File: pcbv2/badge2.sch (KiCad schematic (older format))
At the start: 25 parts, among them J1 Conn_02x04_Counter_Clockwise, J2 SAO_CONN, J3 USB_C_Receptacle_USB2.0, J6 Conn_ARM_JTAG_SWD_10, Q2 Si1308EDL, U3 E73-2G4M08S1C, U5 GD25Q16C, U7 LIS2DH12TR

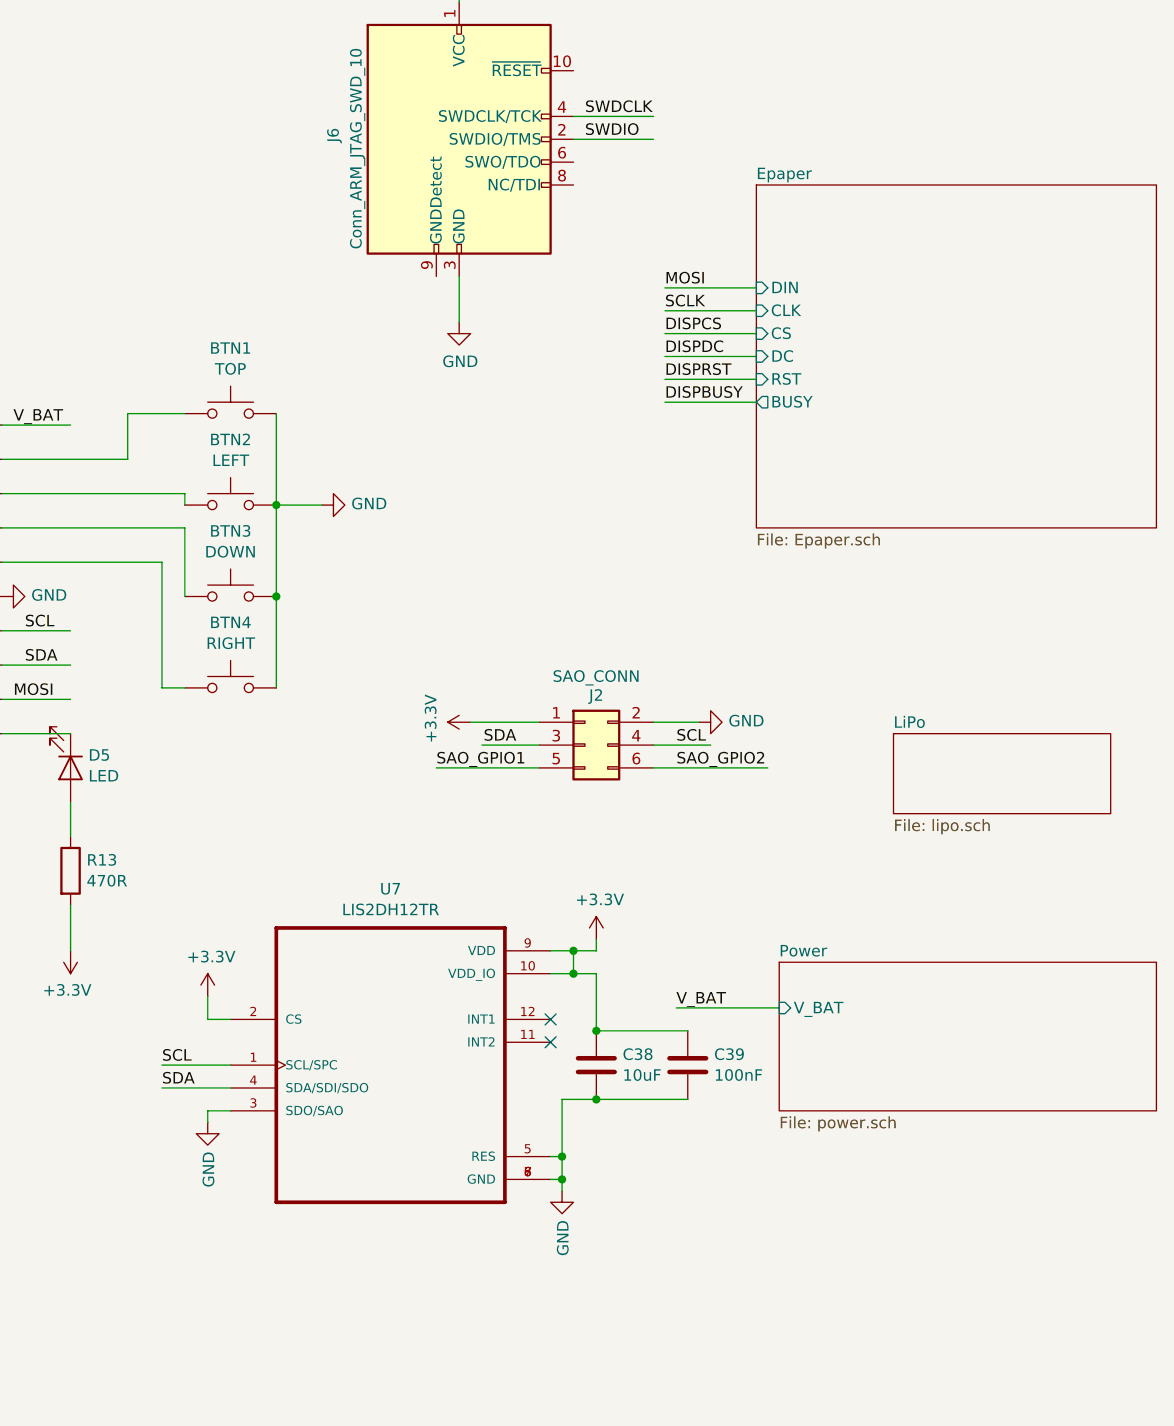
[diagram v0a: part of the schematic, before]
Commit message: refactor(pcbv2): move accelerometer to own sheet
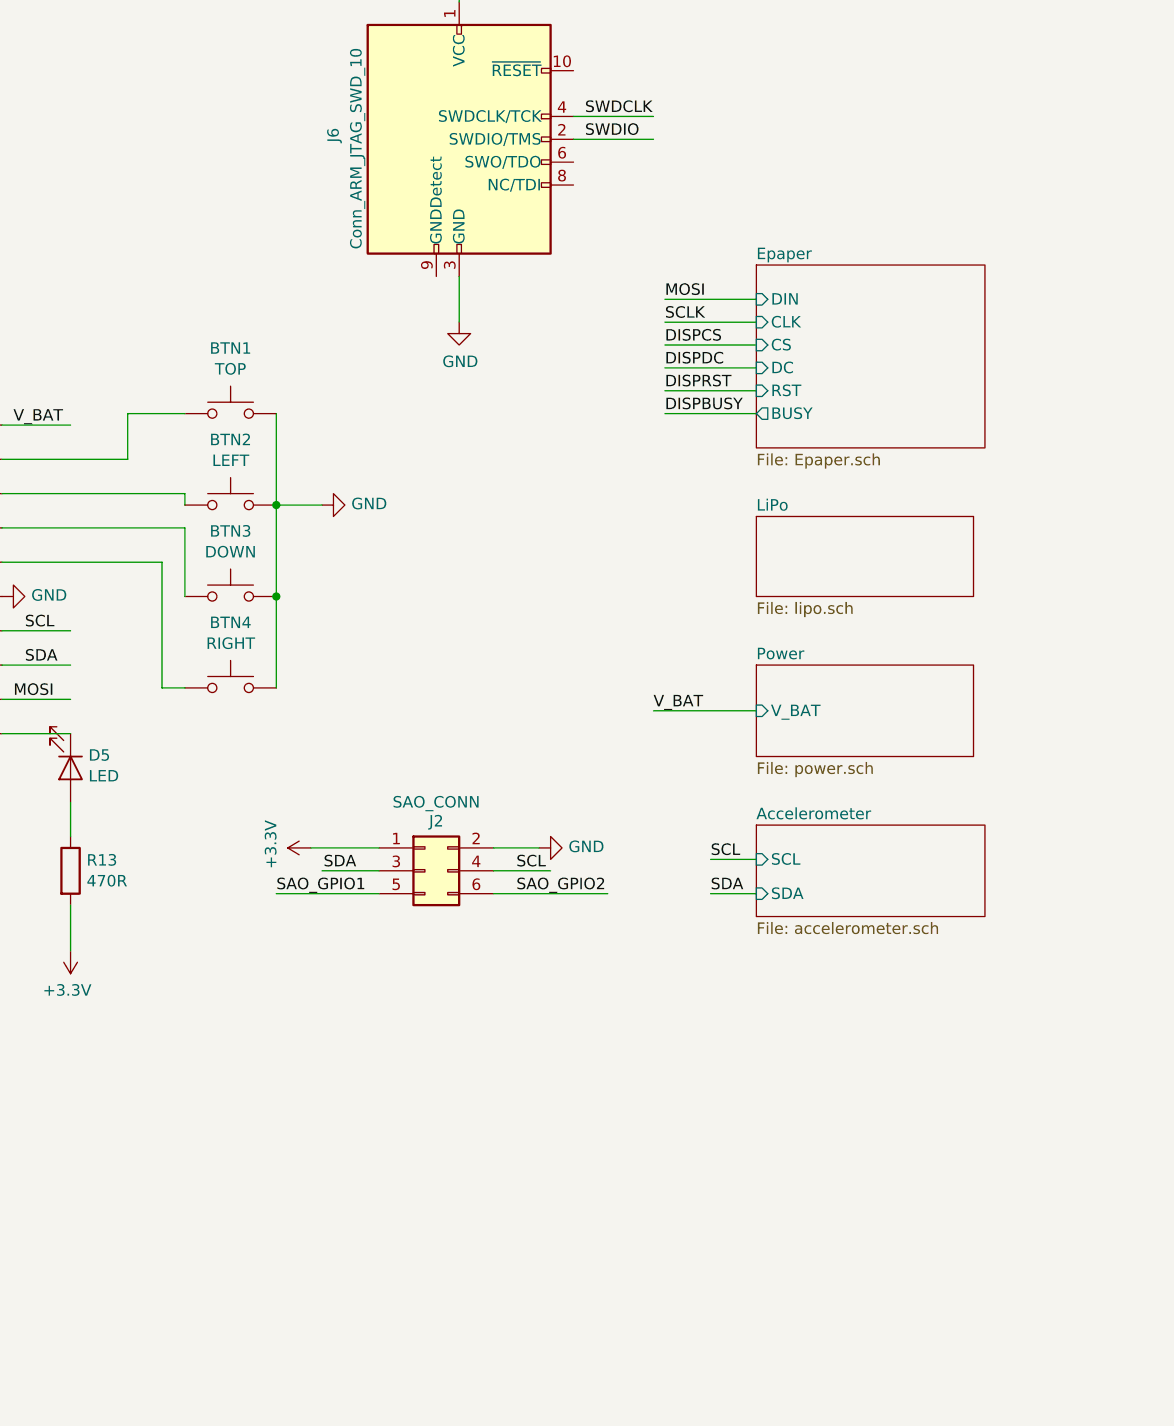
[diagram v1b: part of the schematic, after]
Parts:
- removed C38: 10uF, Capacitor_SMD:C_0603_1608Metric, symbol Device:C
- removed C39: 100nF, Capacitor_SMD:C_0603_1608Metric, symbol Device:C
- removed U7: LIS2DH12TR, Package_LGA:LGA-12_2x2mm_P0.5mm, symbol LIS2DH12TR:LIS2DH12TR
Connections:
- wire segments 134 -> 115
- no-connect marks 6 -> 4
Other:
- moved on the sheet: J2
